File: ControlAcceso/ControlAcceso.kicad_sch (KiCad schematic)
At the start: 7 parts, among them J1 Conn_01x03, J2 Conn_01x07

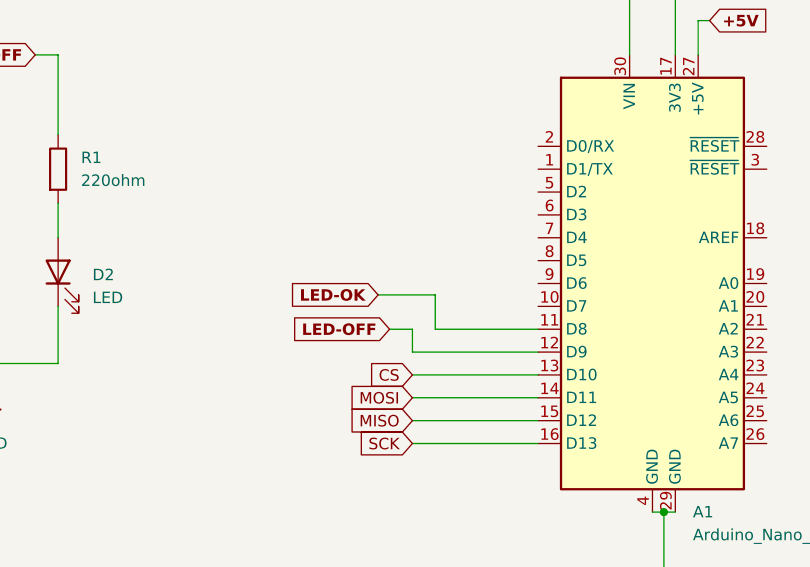
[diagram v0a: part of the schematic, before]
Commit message: Cambios
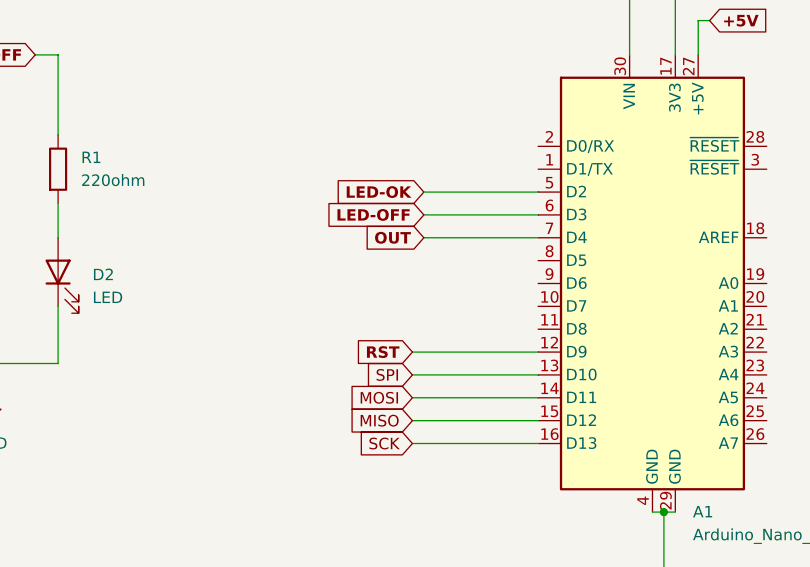
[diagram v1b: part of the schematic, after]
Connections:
- net LED-OFF: now also A1.6 (D3); no longer A1.12 (D9)
- net LED-OK: now also A1.5 (D2); no longer A1.11 (D8)
- net OUT: now also A1.7 (D4)
- net CS renamed SPI
- new net RST: A1.12 (D9)
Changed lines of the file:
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@@
   (junction (at 146.05 97.79) (diameter 0) (color 0 0 0 0)
   )
-  (wire (pts (xy 132.08 77.47) (xy 120.65 77.47))
-    (stroke (width 0) (type default))
-  )
   (wire (pts (xy 186.69 49.53) (xy 187.96 49.53))
     (stroke (width 0) (type default))
   )
+  (wire (pts (xy 119.38 64.77) (xy 132.08 64.77))
+    (stroke (width 0) (type default))
+  )
   (wire (pts (xy 71.12 81.28) (xy 78.74 81.28))
     (stroke (width 0) (type default))
@@
     (stroke (width 0) (type default))
   )
+  (wire (pts (xy 118.11 80.01) (xy 132.08 80.01))
+    (stroke (width 0) (type default))
+  )
   (wire (pts (xy 62.23 81.28) (xy 71.12 81.28))
     (stroke (width 0) (type default))
@@
     (stroke (width 0) (type default))
   )
-  (wire (pts (xy 118.11 77.47) (xy 115.57 77.47))
+  (wire (pts (xy 119.38 67.31) (xy 132.08 67.31))
     (stroke (width 0) (type default))
   )
@@
     (stroke (width 0) (type default))
   )
-  (wire (pts (xy 132.08 80.01) (xy 118.11 80.01))
-    (stroke (width 0) (type default))
-  )
-  (wire (pts (xy 118.11 80.01) (xy 118.11 77.47))
-    (stroke (width 0) (type default))
-  )
   (wire (pts (xy 62.23 63.5) (xy 62.23 67.31))
     (stroke (width 0) (type default))
@@
     (stroke (width 0) (type default))
   )
-  (wire (pts (xy 120.65 77.47) (xy 120.65 73.66))
-    (stroke (width 0) (type default))
-  )
   (wire (pts (xy 193.04 53.34) (xy 186.69 53.34))
     (stroke (width 0) (type default))
@@
     (stroke (width 0) (type default))
   )
-  (wire (pts (xy 120.65 73.66) (xy 114.3 73.66))
+  (wire (pts (xy 119.38 62.23) (xy 132.08 62.23))
     (stroke (width 0) (type default))
   )
@@
     (effects (font (size 2 2) (thickness 0.254) bold) (justify left bottom))
   )
-  (global_label "CS" (shape input) (at 118.11 82.55 180) (fields_autoplaced)
+  (global_label "SPI" (shape input) (at 118.11 82.55 180) (fields_autoplaced)
     (effects (font (size 1.27 1.27)) (justify right))
-    (property "Intersheetrefs" "${INTERSHEET_REFS}" (at 112.7247 82.55 0)
+    (property "Intersheetrefs" "${INTERSHEET_REFS}" (at 112.1199 82.55 0)
       (effects (font (size 1.27 1.27)) (justify right) hide)
     )
@@
     )
   )
+  (global_label "OUT" (shape input) (at 119.38 67.31 180) (fields_autoplaced)
+    (effects (font (size 1.27 1.27) bold) (justify right))
+    (property "Intersheetrefs" "${INTERSHEET_REFS}" (at 112.4172 67.31 0)
+      (effects (font (size 1.27 1.27)) (justify right) hide)
+    )
+  )
   (global_label "LED-OFF" (shape input) (at 76.2 46.99 180) (fields_autoplaced)
     (effects (font (size 1.27 1.27) bold) (justify right))
@@
     )
   )
-  (global_label "LED-OK" (shape input) (at 114.3 73.66 180) (fields_autoplaced)
-    (effects (font (size 1.27 1.27) bold) (justify right))
-    (property "Intersheetrefs" "${INTERSHEET_REFS}" (at 103.3458 73.66 0)
+  (global_label "LED-OK" (shape input) (at 119.38 62.23 180) (fields_autoplaced)
+    (effects (font (size 1.27 1.27) bold) (justify right))
+    (property "Intersheetrefs" "${INTERSHEET_REFS}" (at 108.4258 62.23 0)
       (effects (font (size 1.27 1.27)) (justify right) hide)
     )
@@
     )
   )
-  (global_label "LED-OFF" (shape input) (at 115.57 77.47 180) (fields_autoplaced)
-    (effects (font (size 1.27 1.27) bold) (justify right))
-    (property "Intersheetrefs" "${INTERSHEET_REFS}" (at 103.7086 77.47 0)
+  (global_label "LED-OFF" (shape input) (at 119.38 64.77 180) (fields_autoplaced)
+    (effects (font (size 1.27 1.27) bold) (justify right))
+    (property "Intersheetrefs" "${INTERSHEET_REFS}" (at 107.5186 64.77 0)
       (effects (font (size 1.27 1.27)) (justify right) hide)
     )
@@
     )
   )
+  (global_label "RST" (shape input) (at 118.11 80.01 180) (fields_autoplaced)
+    (effects (font (size 1.27 1.27) bold) (justify right))
+    (property "Intersheetrefs" "${INTERSHEET_REFS}" (at 111.3287 80.01 0)
+      (effects (font (size 1.27 1.27)) (justify right) hide)
+    )
+  )

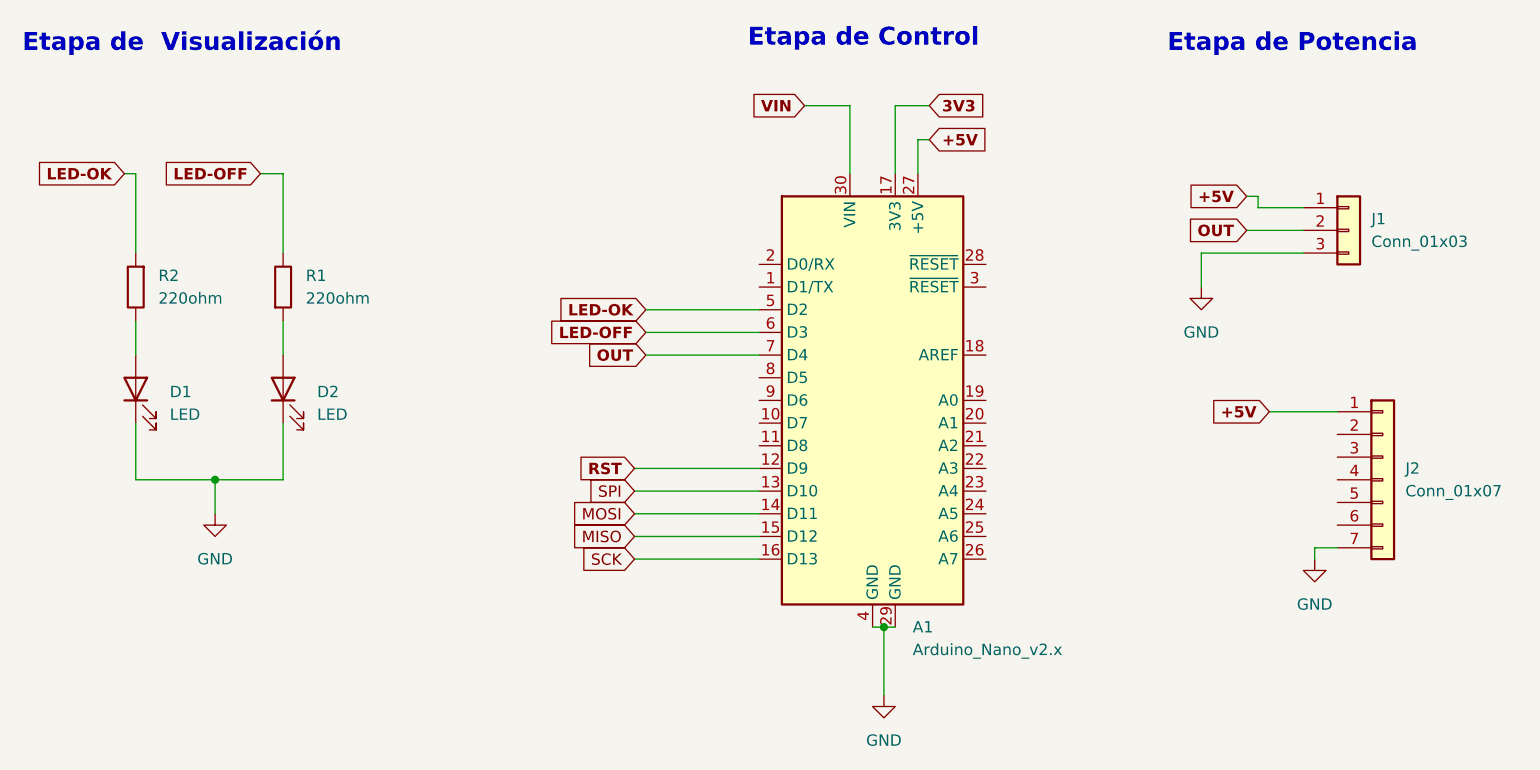
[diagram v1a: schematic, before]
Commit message: Ultimo
Generación de archivos GERBER, modificacion de rutas
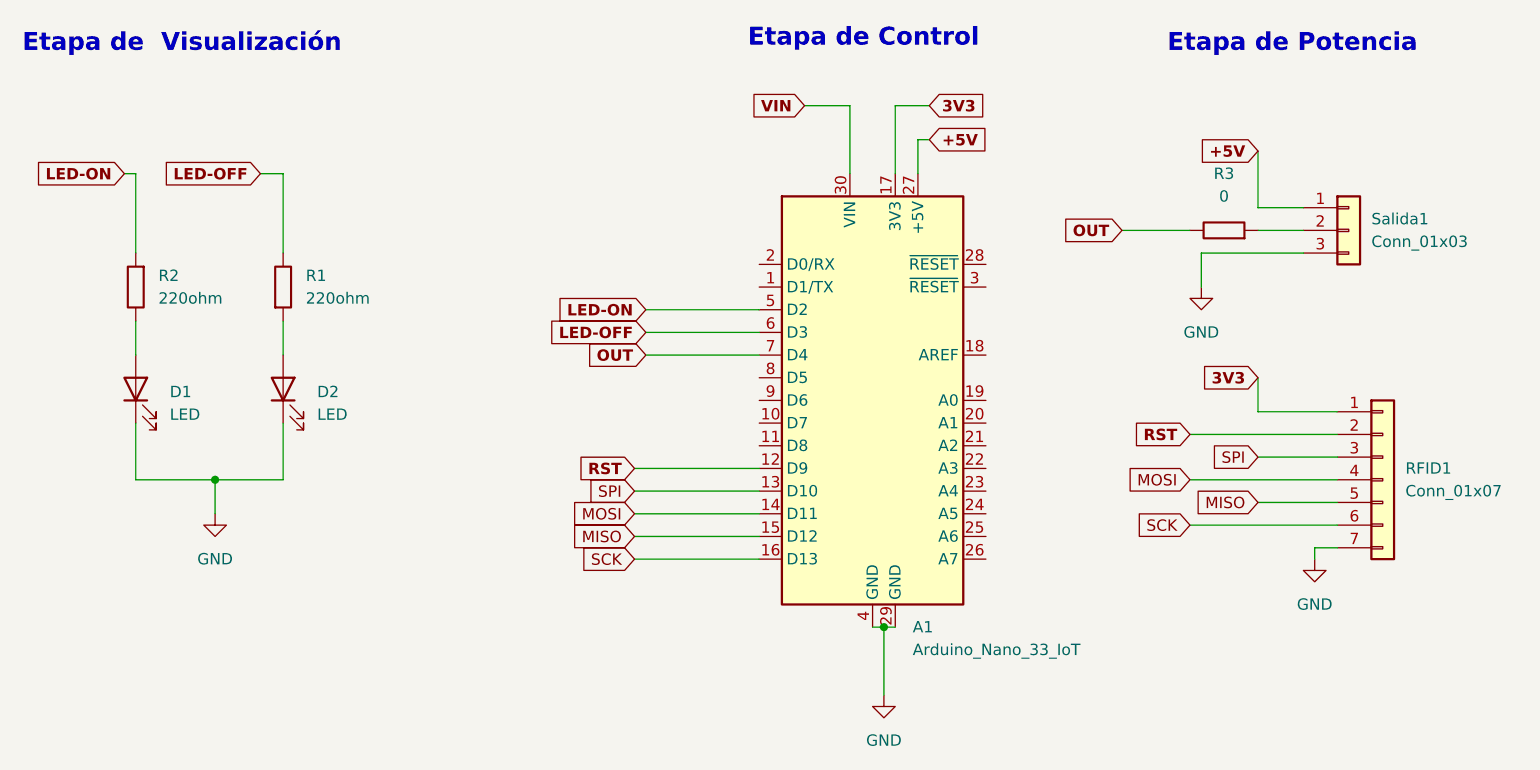
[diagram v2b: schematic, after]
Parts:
- added R3: 0, Resistor_THT:R_Axial_DIN0207_L6.3mm_D2.5mm_P10.16mm_Horizontal, symbol PCM_SL_Resistors:220ohm
- A1: value Arduino_Nano_v2.x -> Arduino_Nano_33_IoT
- D2: footprint (none) -> LED_THT:LED_D5.0mm
- renumbered J2 to RFID1, J1 to Salida1
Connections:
- net +5V: no longer RFID1.1 (Pin_1)
- net 3V3: now also RFID1.1 (Pin_1)
- net MISO: now also RFID1.5 (Pin_5)
- net MOSI: now also RFID1.4 (Pin_4)
- net OUT: now also R3.2; no longer Salida1.2 (Pin_2)
- net RST: now also RFID1.2 (Pin_2)
- net SCK: now also RFID1.6 (Pin_6)
- net SPI: now also RFID1.3 (Pin_3)
- net LED-OK renamed LED-ON
- new net: R3.1, Salida1.2 (Pin_2)
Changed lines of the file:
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@@
   (junction (at 146.05 97.79) (diameter 0) (color 0 0 0 0)
   )
-  (wire (pts (xy 186.69 49.53) (xy 187.96 49.53))
-    (stroke (width 0) (type default))
-  )
   (wire (pts (xy 119.38 64.77) (xy 132.08 64.77))
     (stroke (width 0) (type default))
@@
     (stroke (width 0) (type default))
   )
-  (wire (pts (xy 189.23 73.66) (xy 196.85 73.66))
+  (wire (pts (xy 187.96 73.66) (xy 196.85 73.66))
     (stroke (width 0) (type default))
   )
@@
     (stroke (width 0) (type default))
   )
+  (wire (pts (xy 193.04 53.34) (xy 187.96 53.34))
+    (stroke (width 0) (type default))
+  )
   (wire (pts (xy 119.38 67.31) (xy 132.08 67.31))
     (stroke (width 0) (type default))
@@
     (stroke (width 0) (type default))
   )
+  (wire (pts (xy 196.85 76.2) (xy 180.34 76.2))
+    (stroke (width 0) (type default))
+  )
   (wire (pts (xy 147.32 46.99) (xy 147.32 39.37))
     (stroke (width 0) (type default))
@@
     (stroke (width 0) (type default))
   )
-  (wire (pts (xy 187.96 49.53) (xy 187.96 50.8))
+  (wire (pts (xy 187.96 44.45) (xy 187.96 50.8))
     (stroke (width 0) (type default))
   )
@@
     (stroke (width 0) (type default))
   )
+  (wire (pts (xy 180.34 53.34) (xy 172.72 53.34))
+    (stroke (width 0) (type default))
+  )
   (wire (pts (xy 147.32 39.37) (xy 151.13 39.37))
     (stroke (width 0) (type default))
   )
+  (wire (pts (xy 196.85 86.36) (xy 180.34 86.36))
+    (stroke (width 0) (type default))
+  )
+  (wire (pts (xy 196.85 83.82) (xy 187.96 83.82))
+    (stroke (width 0) (type default))
+  )
   (wire (pts (xy 193.04 55.88) (xy 181.61 55.88))
     (stroke (width 0) (type default))
   )
+  (wire (pts (xy 196.85 78.74) (xy 187.96 78.74))
+    (stroke (width 0) (type default))
+  )
   (wire (pts (xy 144.78 97.79) (xy 146.05 97.79))
     (stroke (width 0) (type default))
   )
-  (wire (pts (xy 193.04 53.34) (xy 186.69 53.34))
+  (wire (pts (xy 196.85 81.28) (xy 180.34 81.28))
+    (stroke (width 0) (type default))
+  )
+  (wire (pts (xy 187.96 69.85) (xy 187.96 73.66))
     (stroke (width 0) (type default))
   )
@@
     )
   )
-  (global_label "OUT" (shape input) (at 186.69 53.34 180) (fields_autoplaced)
-    (effects (font (size 1.27 1.27) bold) (justify right))
-    (property "Intersheetrefs" "${INTERSHEET_REFS}" (at 179.7272 53.34 0)
+  (global_label "OUT" (shape input) (at 172.72 53.34 180) (fields_autoplaced)
+    (effects (font (size 1.27 1.27) bold) (justify right))
+    (property "Intersheetrefs" "${INTERSHEET_REFS}" (at 165.7572 53.34 0)
       (effects (font (size 1.27 1.27)) (justify right) hide)
     )
@@
     )
   )
-  (global_label "+5V" (shape input) (at 189.23 73.66 180) (fields_autoplaced)
-    (effects (font (size 1.27 1.27) bold) (justify right))
-    (property "Intersheetrefs" "${INTERSHEET_REFS}" (at 182.0253 73.66 0)
-      (effects (font (size 1.27 1.27)) (justify right) hide)
-    )
-  )
-  (global_label "LED-OK" (shape input) (at 119.38 62.23 180) (fields_autoplaced)
-    (effects (font (size 1.27 1.27) bold) (justify right))
-    (property "Intersheetrefs" "${INTERSHEET_REFS}" (at 108.4258 62.23 0)
-      (effects (font (size 1.27 1.27)) (justify right) hide)
-    )
-  )
-  (global_label "+5V" (shape input) (at 186.69 49.53 180) (fields_autoplaced)
-    (effects (font (size 1.27 1.27) bold) (justify right))
-    (property "Intersheetrefs" "${INTERSHEET_REFS}" (at 179.4853 49.53 0)
-      (effects (font (size 1.27 1.27)) (justify right) hide)
-    )
-  )
-  (global_label "LED-OK" (shape input) (at 60.96 46.99 180) (fields_autoplaced)
-    (effects (font (size 1.27 1.27) bold) (justify right))
-    (property "Intersheetrefs" "${INTERSHEET_REFS}" (at 50.0058 46.99 0)
+  (global_label "LED-ON" (shape input) (at 119.38 62.23 180) (fields_autoplaced)
+    (effects (font (size 1.27 1.27) bold) (justify right))
+    (property "Intersheetrefs" "${INTERSHEET_REFS}" (at 108.2383 62.23 0)
+      (effects (font (size 1.27 1.27)) (justify right) hide)
+    )
+  )
+  (global_label "SCK" (shape input) (at 180.34 86.36 180) (fields_autoplaced)
+    (effects (font (size 1.27 1.27)) (justify right))
+    (property "Intersheetrefs" "${INTERSHEET_REFS}" (at 173.6847 86.36 0)
+      (effects (font (size 1.27 1.27)) (justify right) hide)
+    )
+  )
+  (global_label "SPI" (shape input) (at 187.96 78.74 180) (fields_autoplaced)
+    (effects (font (size 1.27 1.27)) (justify right))
+    (property "Intersheetrefs" "${INTERSHEET_REFS}" (at 181.9699 78.74 0)
+      (effects (font (size 1.27 1.27)) (justify right) hide)
+    )
+  )
+  (global_label "MOSI" (shape input) (at 180.34 81.28 180) (fields_autoplaced)
+    (effects (font (size 1.27 1.27)) (justify right))
+    (property "Intersheetrefs" "${INTERSHEET_REFS}" (at 172.838 81.28 0)
+      (effects (font (size 1.27 1.27)) (justify right) hide)
+    )
+  )
+  (global_label "+5V" (shape input) (at 187.96 44.45 180) (fields_autoplaced)
+    (effects (font (size 1.27 1.27) bold) (justify right))
+    (property "Intersheetrefs" "${INTERSHEET_REFS}" (at 180.7553 44.45 0)
+      (effects (font (size 1.27 1.27)) (justify right) hide)
+    )
+  )
+  (global_label "MISO" (shape input) (at 187.96 83.82 180) (fields_autoplaced)
+    (effects (font (size 1.27 1.27)) (justify right))
+    (property "Intersheetrefs" "${INTERSHEET_REFS}" (at 180.458 83.82 0)
+      (effects (font (size 1.27 1.27)) (justify right) hide)
+    )
+  )
+  (global_label "LED-ON" (shape input) (at 60.96 46.99 180) (fields_autoplaced)
+    (effects (font (size 1.27 1.27) bold) (justify right))
+    (property "Intersheetrefs" "${INTERSHEET_REFS}" (at 49.8183 46.99 0)
       (effects (font (size 1.27 1.27)) (justify right) hide)
     )
@@
     )
   )
+  (global_label "RST" (shape input) (at 180.34 76.2 180) (fields_autoplaced)
+    (effects (font (size 1.27 1.27) bold) (justify right))
+    (property "Intersheetrefs" "${INTERSHEET_REFS}" (at 173.5587 76.2 0)
+      (effects (font (size 1.27 1.27)) (justify right) hide)
+    )
+  )
   (global_label "RST" (shape input) (at 118.11 80.01 180) (fields_autoplaced)
     (effects (font (size 1.27 1.27) bold) (justify right))
@@
     (effects (font (size 1.27 1.27)) (justify right))
     (property "Intersheetrefs" "${INTERSHEET_REFS}" (at 111.4547 90.17 0)
+      (effects (font (size 1.27 1.27)) (justify right) hide)
+    )
+  )
+  (global_label "3V3" (shape input) (at 187.96 69.85 180) (fields_autoplaced)
+    (effects (font (size 1.27 1.27) bold) (justify right))
+    (property "Intersheetrefs" "${INTERSHEET_REFS}" (at 181.1182 69.85 0)
       (effects (font (size 1.27 1.27)) (justify right) hide)
     )
@@
       (effects (font (size 1.27 1.27)) (justify right))
     )
-    (property "Footprint" "" (at 78.74 71.12 0)
+    (property "Footprint" "LED_THT:LED_D5.0mm" (at 78.74 71.12 0)
       (effects (font (size 1.27 1.27)) hide)
     )
@@
         (path "/01db9da7-ae97-4914-ace0-84de2f5ab849"
           (reference "D2") (unit 1)
+        )
+      )
+    )
+  )
+  (symbol (lib_id "PCM_SL_Resistors:220ohm") (at 184.15 53.34 180) (unit 1)
+    (in_bom yes) (on_board yes) (dnp no) (fields_autoplaced)
+    (property "Reference" "R3" (at 184.15 46.99 0)
+      (effects (font (size 1.27 1.27)))
+    )
+    (property "Value" "0" (at 184.15 49.53 0)
+      (effects (font (size 1.27 1.27)))
+    )
+    (property "Footprint" "Resistor_THT:R_Axial_DIN0207_L6.3mm_D2.5mm_P10.16mm_Horizontal" (at 183.261 49.022 0)
+      (effects (font (size 1.27 1.27)) hide)
+    )
+    (property "Datasheet" "" (at 183.642 53.34 0)
+      (effects (font (size 1.27 1.27)) hide)
+    )
+    (pin "1")
+    (pin "2")
+    (instances
+      (project "ControlAcceso"
+        (path "/01db9da7-ae97-4914-ace0-84de2f5ab849"
+          (reference "R3") (unit 1)
         )
       )
@@
       (effects (font (size 1.27 1.27)) (justify left))
     )
-    (property "Value" "Arduino_Nano_v2.x" (at 149.2759 100.33 0)
+    (property "Value" "Arduino_Nano_33_IoT" (at 149.2759 100.33 0)
       (effects (font (size 1.27 1.27)) (justify left))
     )
@@
   (symbol (lib_id "Connector_Generic:Conn_01x07") (at 201.93 81.28 0) (unit 1)
     (in_bom yes) (on_board yes) (dnp no) (fields_autoplaced)
-    (property "Reference" "J2" (at 204.47 80.01 0)
+    (property "Reference" "RFID1" (at 204.47 80.01 0)
       (effects (font (size 1.27 1.27)) (justify left))
     )
@@
       (project "ControlAcceso"
         (path "/01db9da7-ae97-4914-ace0-84de2f5ab849"
-          (reference "J2") (unit 1)
+          (reference "RFID1") (unit 1)
         )
       )
@@
   (symbol (lib_id "PCM_4ms_Connector:Conn_01x03") (at 198.12 53.34 0) (unit 1)
     (in_bom yes) (on_board yes) (dnp no) (fields_autoplaced)
-    (property "Reference" "J1" (at 200.66 52.07 0)
+    (property "Reference" "Salida1" (at 200.66 52.07 0)
       (effects (font (size 1.27 1.27)) (justify left))
     )
@@
       (project "ControlAcceso"
         (path "/01db9da7-ae97-4914-ace0-84de2f5ab849"
-          (reference "J1") (unit 1)
-        )
-      )
+          (reference "Salida1") (unit 1)
+        )
+      )
